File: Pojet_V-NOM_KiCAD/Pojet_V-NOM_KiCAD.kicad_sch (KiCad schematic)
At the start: 4 parts

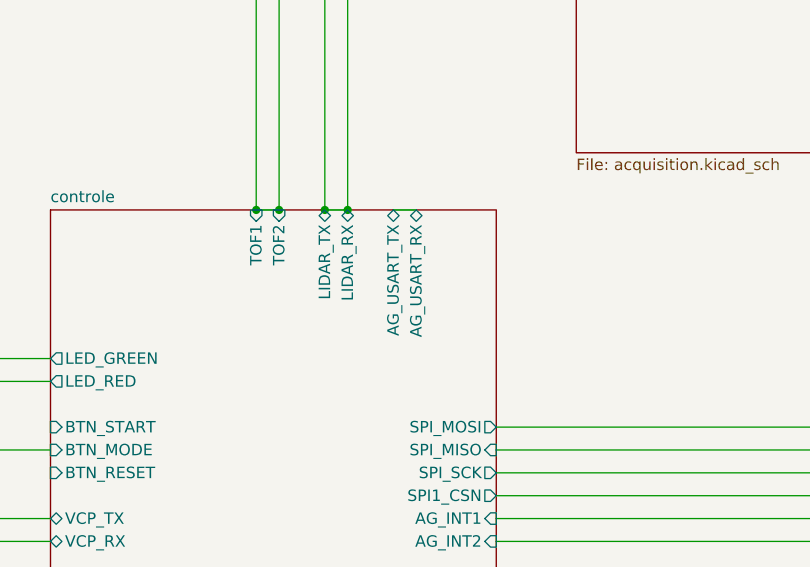
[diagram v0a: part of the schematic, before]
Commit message: Corrections rapides du schéma global
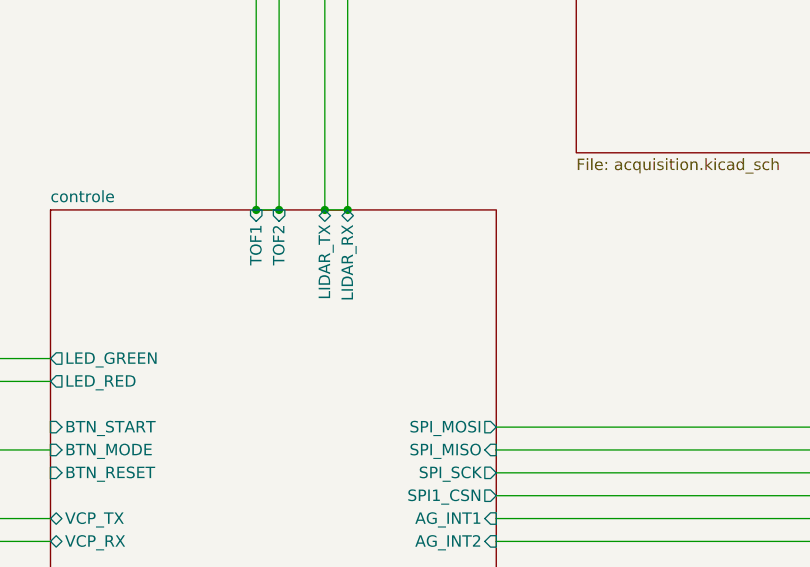
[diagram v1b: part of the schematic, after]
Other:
- sheet controle ports: added none; removed AG_USART_RX, AG_USART_TX
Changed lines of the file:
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@@
-	(wire
-		(pts
-			(xy 153.67 71.12) (xy 151.13 71.12)
-		)
-		(stroke
-			(width 0)
-			(type default)
-		)
-	)
 	(wire
 		(pts
@@
 			)
 		)
-		(pin "AG_USART_TX" bidirectional
-			(at 151.13 71.12 90)
-			(effects
-				(font
-					(size 1.27 1.27)
-				)
-				(justify right)
-			)
-		)
 		(pin "TIM3_CH2" output
 			(at 142.24 124.46 270)
@@
 			)
 		)
-		(pin "AG_USART_RX" bidirectional
-			(at 153.67 71.12 90)
-			(effects
-				(font
-					(size 1.27 1.27)
-				)
-				(justify right)
-			)
-		)
